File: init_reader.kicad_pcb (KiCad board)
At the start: 2 copper layers, 95 x 143 mm, 30 parts, among them J1 DE9_Pins, Q1 Q_NPN, SW1 1, SW2 2, SW3 3, SW4 4, U1 LCD_16x4, U2 MAX232, U3 5V, U4 Optocoupler_DC_PhotoNPN_AKEC, U5_MT3608 +24V, U6 AMS1117-3.3

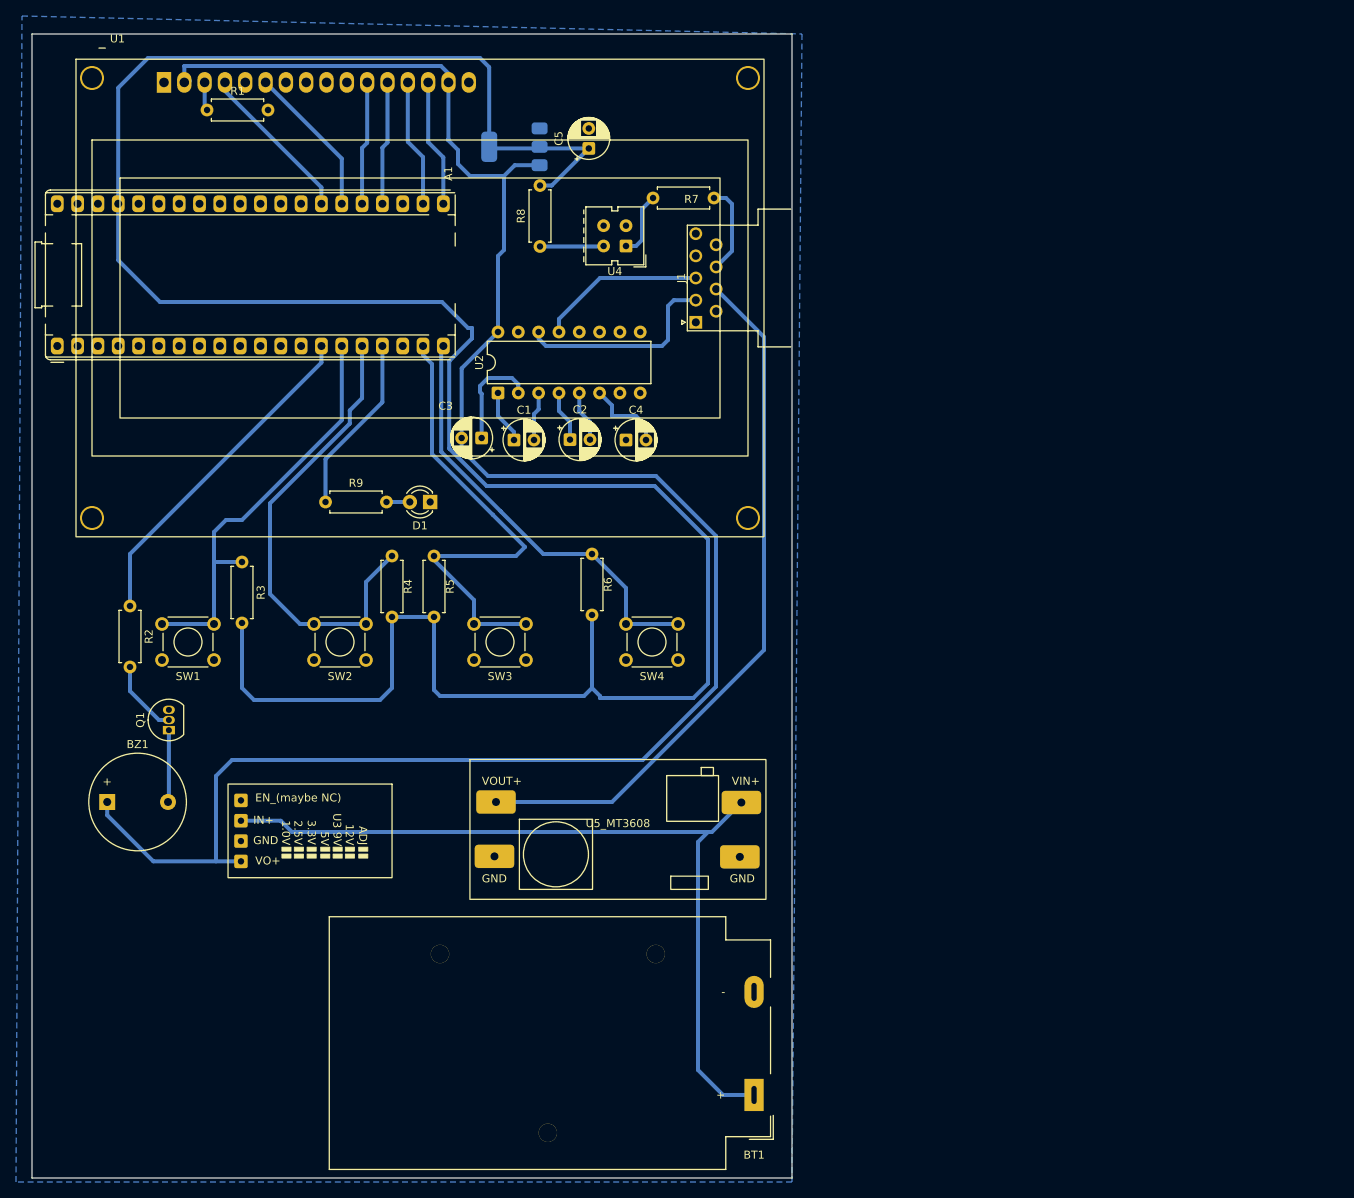
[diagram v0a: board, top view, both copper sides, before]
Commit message: update all
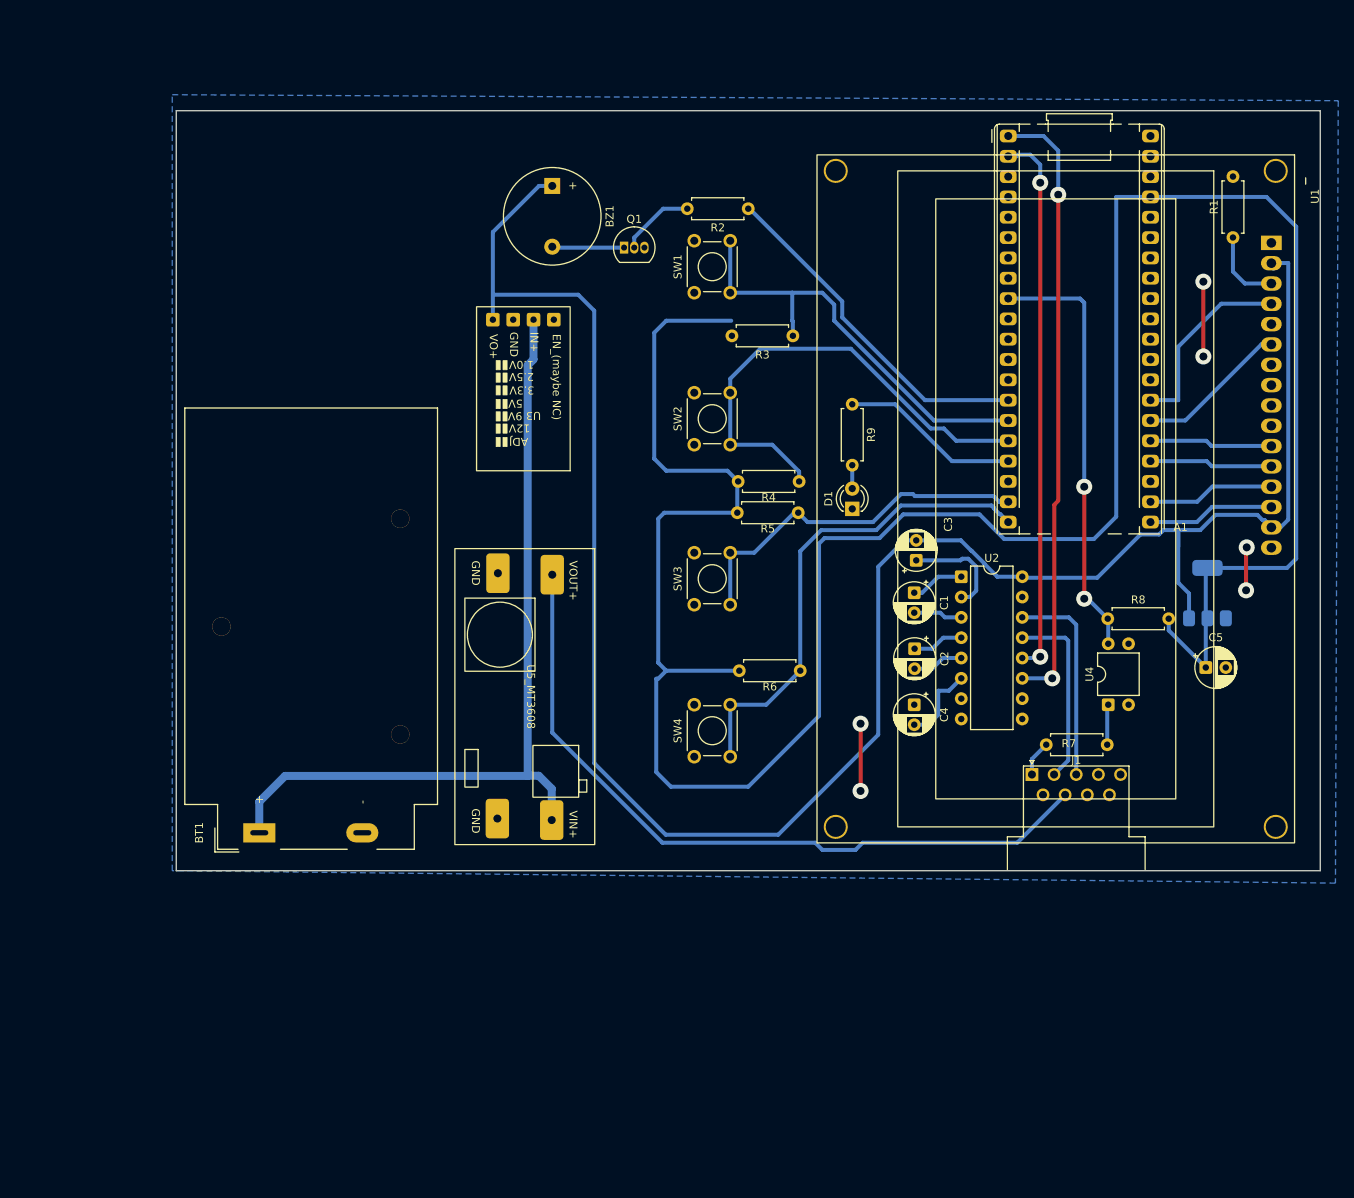
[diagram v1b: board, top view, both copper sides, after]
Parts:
- U4: footprint OptoDevice:Vishay_CNY70 -> Package_DIP:DIP-4_W7.62mm
- moved R1 129.2 mm to (254.1, 43.4), turned to 90 degrees
- moved A1 121.7 mm to (226.0, 30.8), turned to 0 degrees
- moved U6 103.0 mm to (250.9, 87.9), turned to 90 degrees
- moved C5 100.8 mm to (250.7, 97.2), turned to 0 degrees
- moved BZ1 95.0 mm to (169.0, 37.0), turned to -90 degrees
- moved R2 91.9 mm to (193.5, 39.8), turned to 180 degrees
- moved R8 84.9 mm to (238.5, 91.1), turned to 0 degrees
- moved U1 83.3 mm to (232.0, 76.1), turned to -90 degrees
- moved U4 83.2 mm to (238.5, 101.8), turned to 90 degrees
- moved Q1 82.9 mm to (178.0, 44.7), turned to 0 degrees
- moved R7 80.0 mm to (230.8, 106.8), turned to 0 degrees
- moved SW1 75.6 mm to (186.8, 50.3), turned to 90 degrees
- moved R3 74.4 mm to (199.1, 55.7), turned to 180 degrees
- moved J1 70.4 mm to (229.0, 110.6), turned to 0 degrees
- moved BT1 70.0 mm to (132.4, 117.8), turned to 90 degrees
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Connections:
- A1 pad 1: unconnected-(A1-GPIO0-Pad1) -> T1OUT
- A1 pad 2: unconnected-(A1-GPIO1-Pad2) -> R1OUT
- A1 pad 9: unconnected-(A1-GPIO6-Pad9) -> Present_mcu
- J1 pad 1: unconnected-(J1-Pad1) -> Present
- J1 pad 2: T1IN -> R1IN
- J1 pad 3: R1IN -> T1IN
- J1 pad 8: Present -> unconnected-(J1-Pad8)
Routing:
- net T1OUT: track 0.00 -> 77.0 mm, vias 0 -> 2
- net R1OUT: track 0.00 -> 68.4 mm, vias 0 -> 2
- net Present_mcu: track 7.97 -> 53.8 mm, vias 0 -> 2
- net GND: track 0.00 -> 23.3 mm, vias 0 -> 6
- net +5V: track 248.8 -> 263.0 mm
- net GP14: track 59.3 -> 45.7 mm
- net Present: track 11.2 -> 4.47 mm
- net GP15: track 54.5 -> 61.2 mm
- net Net-(U1-VO): track 3.57 -> 9.68 mm
- net RS: track 20.2 -> 24.1 mm
- net +24V: track 89.0 -> 92.8 mm
- net Net-(R7-Pad2): track 8.13 -> 5.05 mm
- net R1IN: track 20.8 -> 23.4 mm
- net +3.3V: track 316.4 -> 318.7 mm
- net GP11: track 52.5 -> 54.5 mm
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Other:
- board size 95 x 143 mm -> 143 x 95 mm
